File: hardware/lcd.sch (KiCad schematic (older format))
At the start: 3 parts

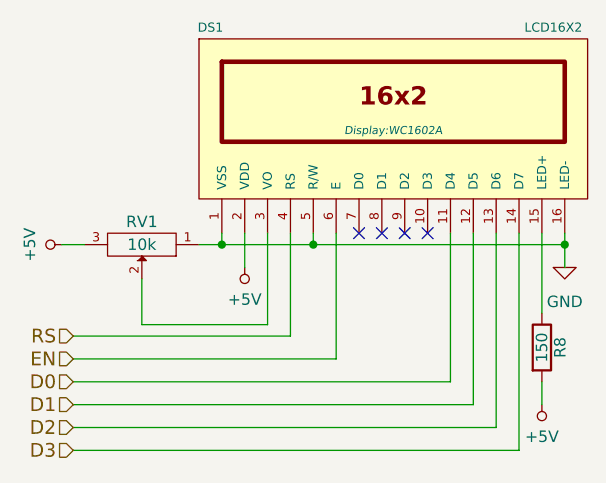
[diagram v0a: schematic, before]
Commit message: diverese Sachen geändert
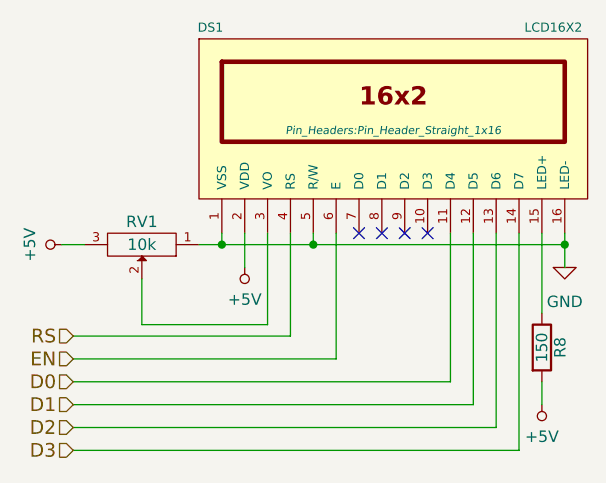
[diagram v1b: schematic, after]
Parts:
- DS1: footprint Display:WC1602A -> Pin_Headers:Pin_Header_Straight_1x16
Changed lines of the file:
@@
 	6850 3350 6850 3500
 $Comp
-L GND #PWR012
+L GND #PWR015
 U 1 1 55F9D0E8
 P 6850 3500
-F 0 "#PWR012" H 6850 3250 50  0001 C CNN
+F 0 "#PWR015" H 6850 3250 50  0001 C CNN
 F 1 "GND" H 6850 3350 50  0000 C CNN
 F 2 "" H 6850 3500 60  0000 C CNN
@@
 F 0 "DS1" H 5300 3250 40  0000 C CNN
 F 1 "LCD16X2" H 6800 3250 40  0000 C CNN
-F 2 "Display:WC1602A" H 6100 2800 35  0000 C CIN
+F 2 "Pin_Headers:Pin_Header_Straight_1x16" H 6100 2800 35  0000 C CIN
 F 3 "" H 6100 2850 60  0000 C CNN
 	1    6100 2850
@@
 Connection ~ 5750 3400
 $Comp
-L +5V #PWR013
+L +5V #PWR016
 U 1 1 55F9F555
 P 5450 3500
-F 0 "#PWR013" H 5450 3350 50  0001 C CNN
+F 0 "#PWR016" H 5450 3350 50  0001 C CNN
 F 1 "+5V" H 5450 3640 50  0000 C CNN
 F 2 "" H 5450 3500 60  0000 C CNN
@@
 	5550 3750 5550 3350
 $Comp
-L +5V #PWR014
+L +5V #PWR017
 U 1 1 55F9F9A0
 P 4650 3400
-F 0 "#PWR014" H 4650 3250 50  0001 C CNN
+F 0 "#PWR017" H 4650 3250 50  0001 C CNN
 F 1 "+5V" H 4650 3540 50  0000 C CNN
 F 2 "" H 4650 3400 60  0000 C CNN
@@
 $EndComp
 $Comp
-L +5V #PWR015
+L +5V #PWR018
 U 1 1 55F9FC92
 P 6750 4100
-F 0 "#PWR015" H 6750 3950 50  0001 C CNN
+F 0 "#PWR018" H 6750 3950 50  0001 C CNN
 F 1 "+5V" H 6750 4240 50  0000 C CNN
 F 2 "" H 6750 4100 60  0000 C CNN
